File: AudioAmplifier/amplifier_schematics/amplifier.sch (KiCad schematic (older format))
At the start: 2 parts

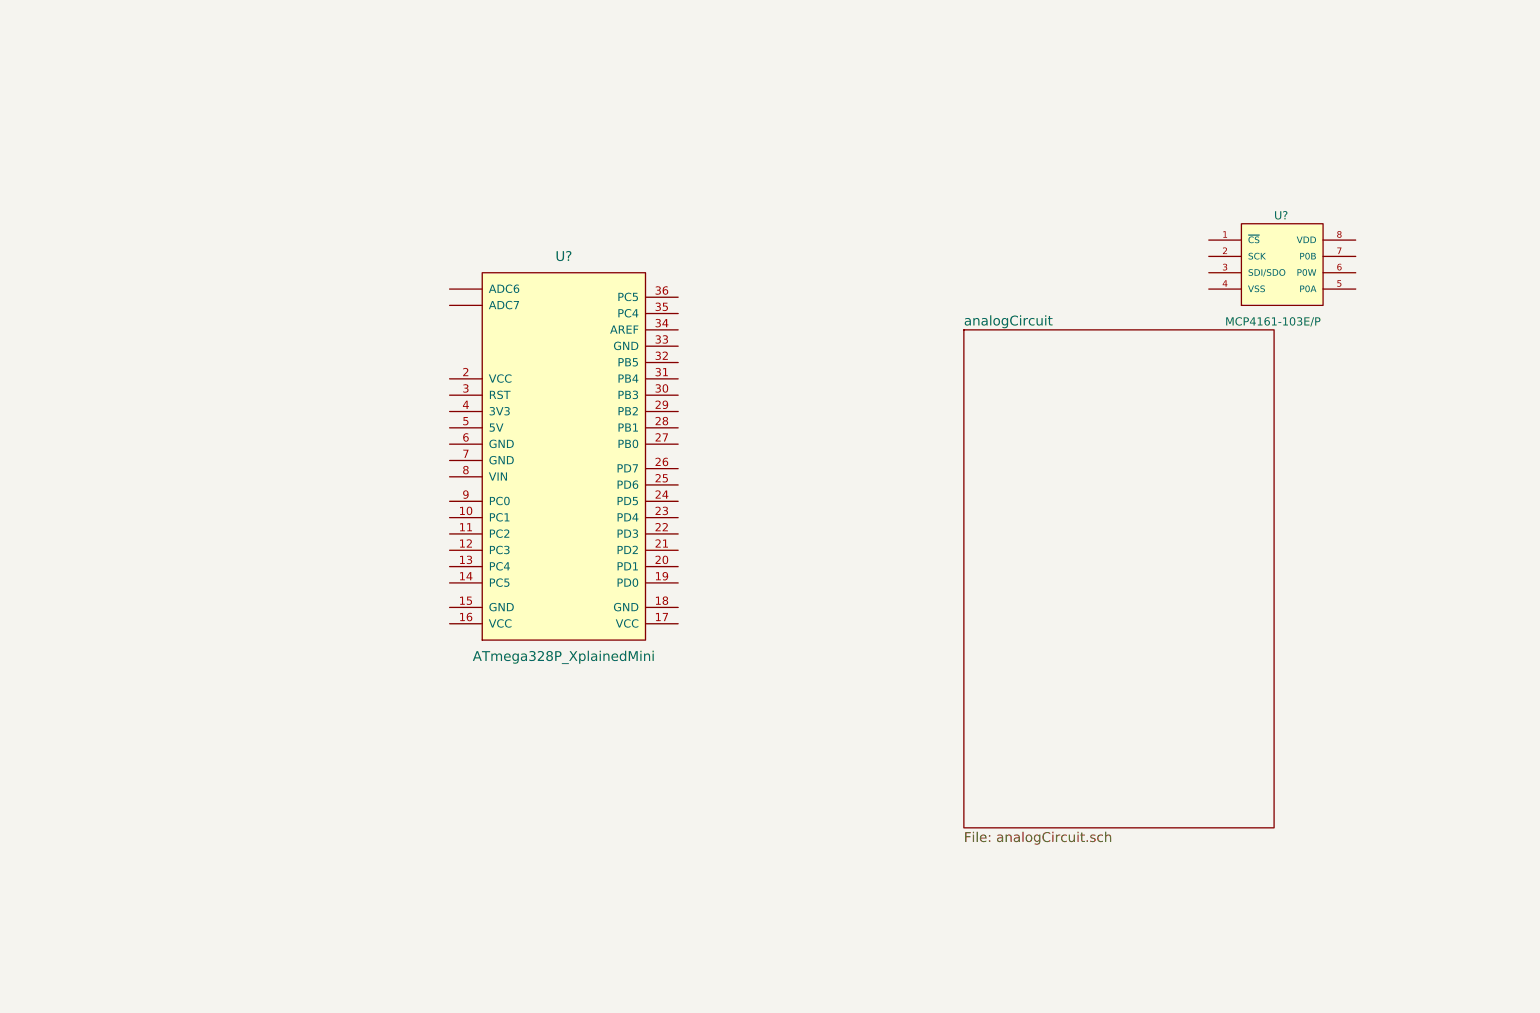
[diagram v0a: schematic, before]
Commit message: updated kicad file
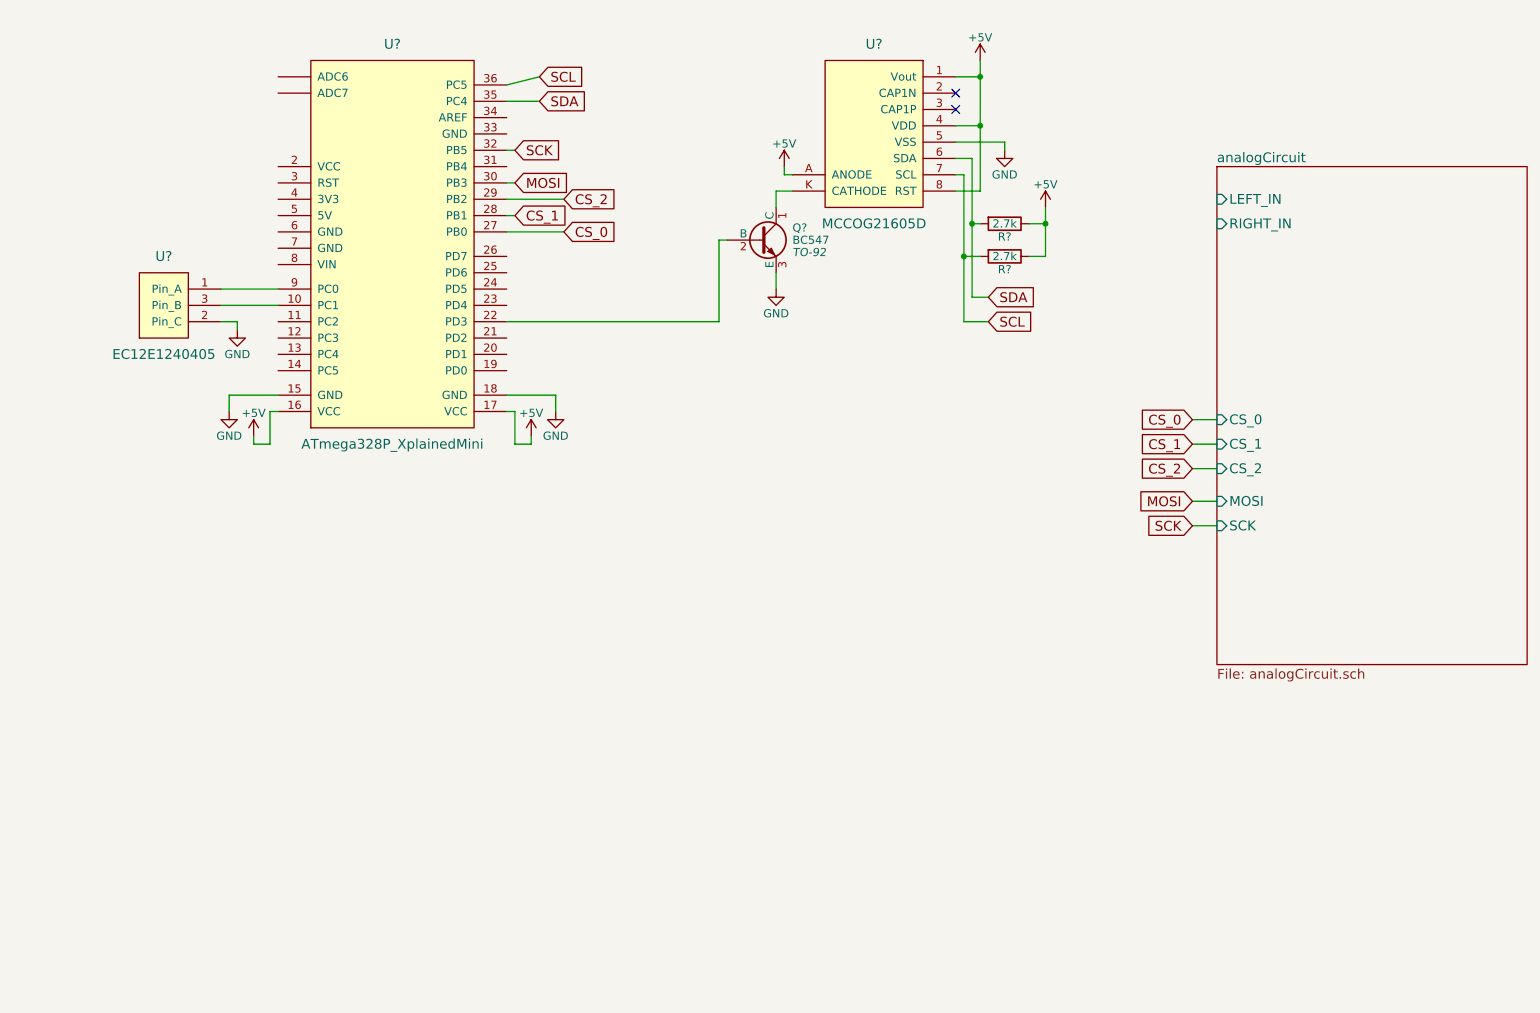
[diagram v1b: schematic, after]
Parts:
- removed U?: MCP4161-103E/P, DIP254P762X533-8, symbol MCP4161-103E/P
- added Q?: BC547, TO-92, symbol BC547
- added R? (x2): 2.7k, symbol R
- added U?: MCCOG21605D, symbol MCCOG21605D
- added U?: EC12E1240405, symbol EC12E1240405
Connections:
- net at U?.10 (PC1): now also U?.3 (Pin_B)
- net GND: now reaches U?.15 (GND)
- net GND: now also U?.18 (GND), Q?.3 (E), U?.2 (Pin_C), U?.5 (VSS)
- net +5V: now reaches U?.16 (VCC)
- net +5V: now also U?.17 (VCC), R?.1, R?.1, U?.1 (Vout), U?.4 (VDD), U?.8 (RST), U?.A (ANODE)
- net at U?.22 (PD3): now also Q?.2 (B)
- net CS_0: now reaches U?.27 (PB0)
- net CS_1: now reaches U?.28 (PB1)
- net CS_2: now reaches U?.29 (PB2)
- net MOSI: now reaches U?.30 (PB3)
- net SCK: now reaches U?.32 (PB5)
- net SDA: now reaches U?.35 (PC4)
- net SDA: now also R?.2, U?.6 (SDA)
- net SCL: now reaches U?.36 (PC5)
- net SCL: now also R?.2, U?.7 (SCL)
- net at U?.9 (PC0): now also U?.1 (Pin_A)
- new net: Q?.1 (C), U?.K (CATHODE)
- no-connect marks 0 -> 2
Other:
- moved on the sheet: U?

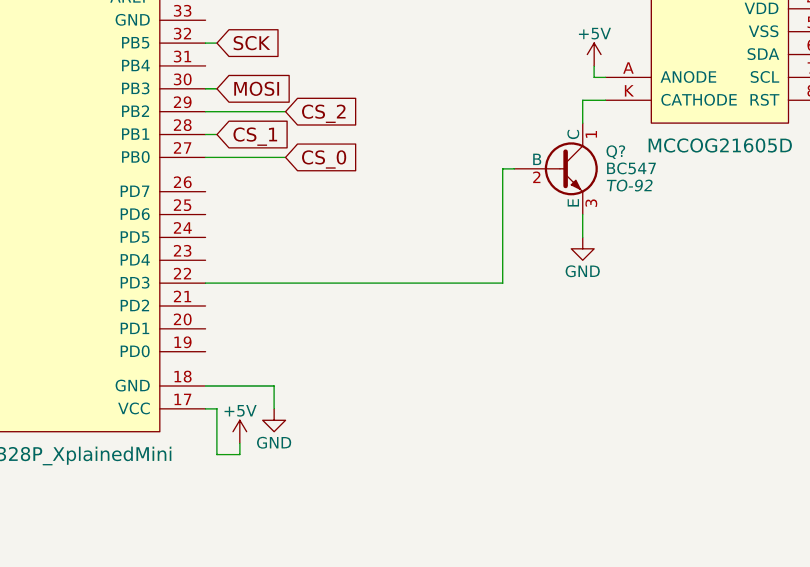
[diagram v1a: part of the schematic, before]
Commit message: kicad schem
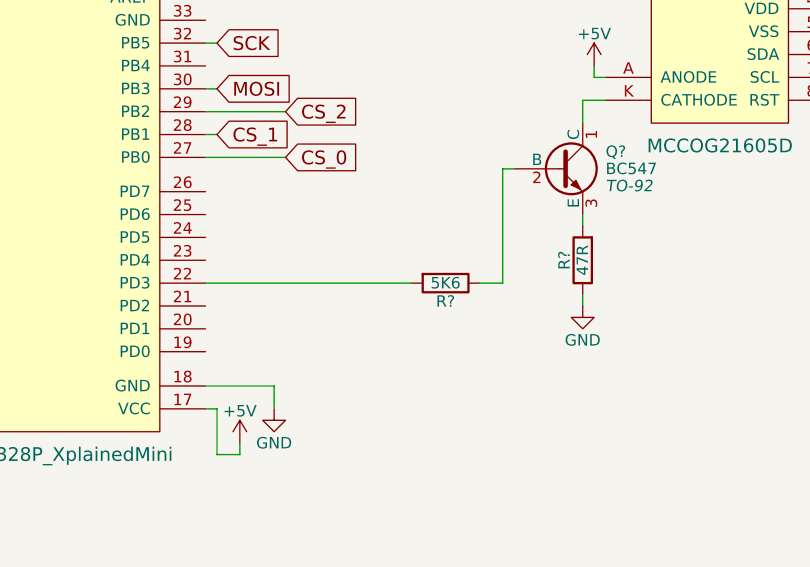
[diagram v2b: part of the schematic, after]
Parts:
- added R?: 5K6, symbol R
- added R?: 47R, symbol R
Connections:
- net GND: now also R?.1; no longer Q?.3 (E)
- net at U?.22 (PD3): now also R?.2; no longer Q?.2 (B)
- new net: Q?.2 (B), R?.1
- new net: Q?.3 (E), R?.2
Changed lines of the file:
@@
 L GND #PWR?
 U 1 1 58FDA342
-P 5200 2900
-F 0 "#PWR?" H 5200 2650 50  0001 C CNN
-F 1 "GND" H 5200 2750 50  0000 C CNN
-F 2 "" H 5200 2900 50  0000 C CNN
-F 3 "" H 5200 2900 50  0000 C CNN
-	1    5200 2900
-	1    0    0    -1
-$EndComp
-Wire Wire Line
-	5200 2800 5200 2900
-Wire Wire Line
-	3550 3100 4850 3100
+P 5200 3200
+F 0 "#PWR?" H 5200 2950 50  0001 C CNN
+F 1 "GND" H 5200 3050 50  0000 C CNN
+F 2 "" H 5200 3200 50  0000 C CNN
+F 3 "" H 5200 3200 50  0000 C CNN
+	1    5200 3200
+	1    0    0    -1
+$EndComp
+Wire Wire Line
+	5200 2800 5200 2850
 Wire Wire Line
 	4850 3100 4850 2600
@@
 Wire Wire Line
 	7750 4350 7900 4350
+$Comp
+L R R?
+U 1 1 5900779A
+P 4600 3100
+F 0 "R?" V 4680 3100 50  0000 C CNN
+F 1 "5K6" V 4600 3100 50  0000 C CNN
+F 2 "" V 4530 3100 50  0000 C CNN
+F 3 "" H 4600 3100 50  0000 C CNN
+	1    4600 3100
+	0    1    1    0
+$EndComp
+$Comp
+L R R?
+U 1 1 5900780C
+P 5200 3000
+F 0 "R?" V 5280 3000 50  0000 C CNN
+F 1 "47R" V 5200 3000 50  0000 C CNN
+F 2 "" V 5130 3000 50  0000 C CNN
+F 3 "" H 5200 3000 50  0000 C CNN
+	1    5200 3000
+	-1   0    0    1
+$EndComp
+Wire Wire Line
+	4750 3100 4850 3100
+Wire Wire Line
+	4450 3100 3550 3100
+Wire Wire Line
+	5200 3150 5200 3200
 $EndSCHEMATC

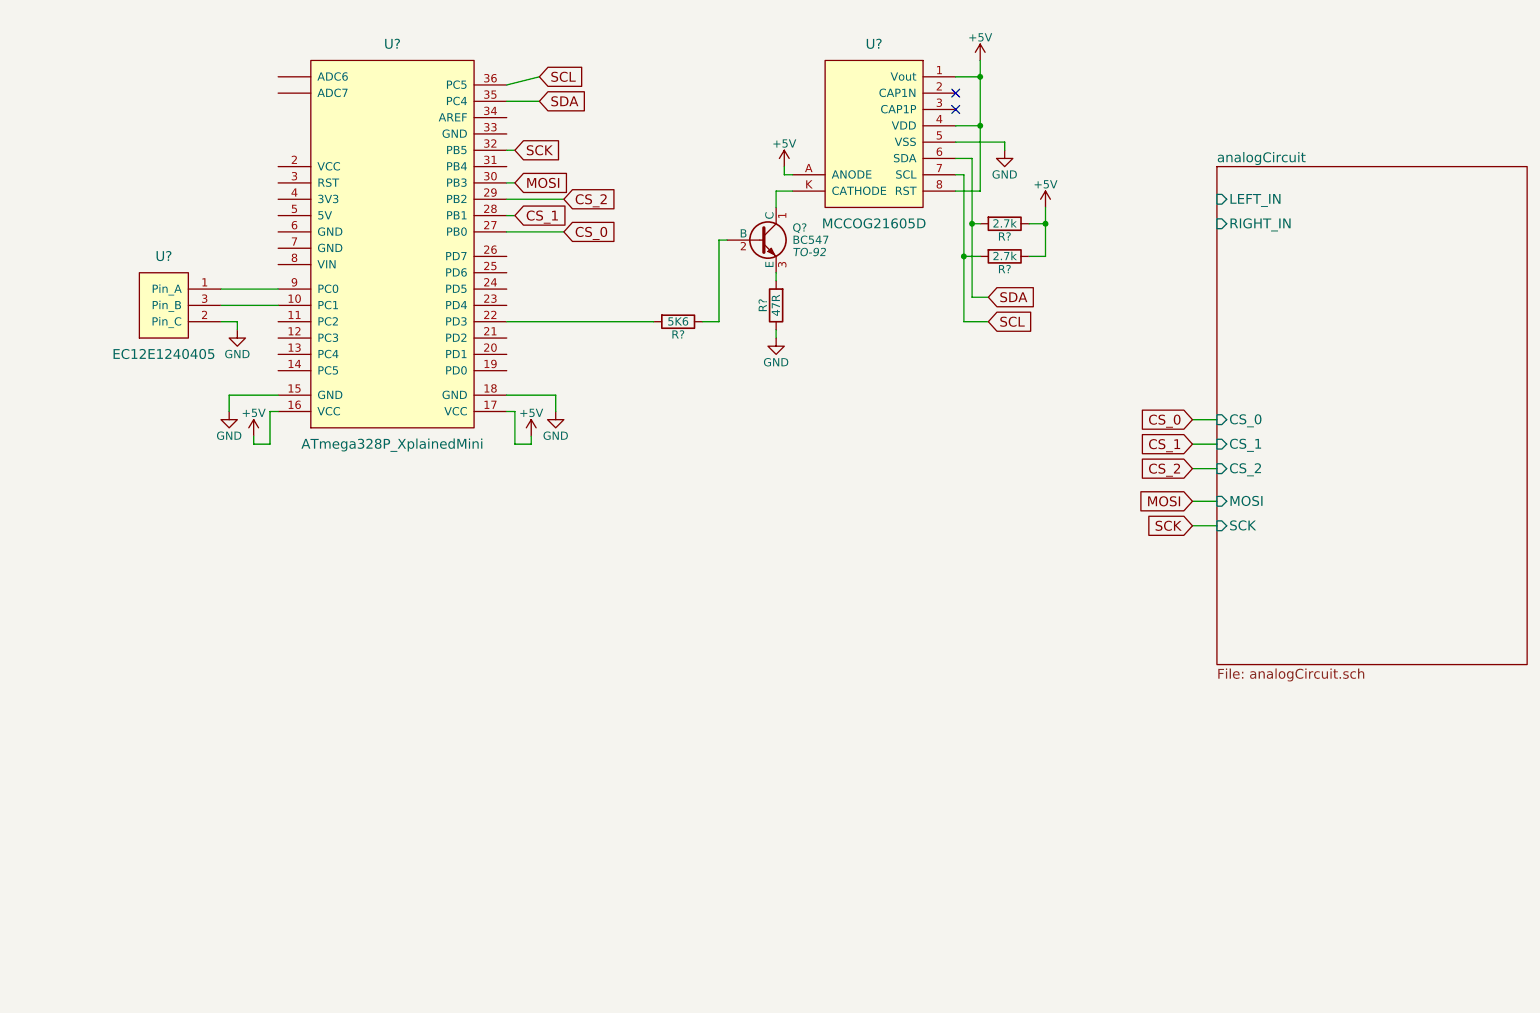
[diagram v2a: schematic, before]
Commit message: kicad
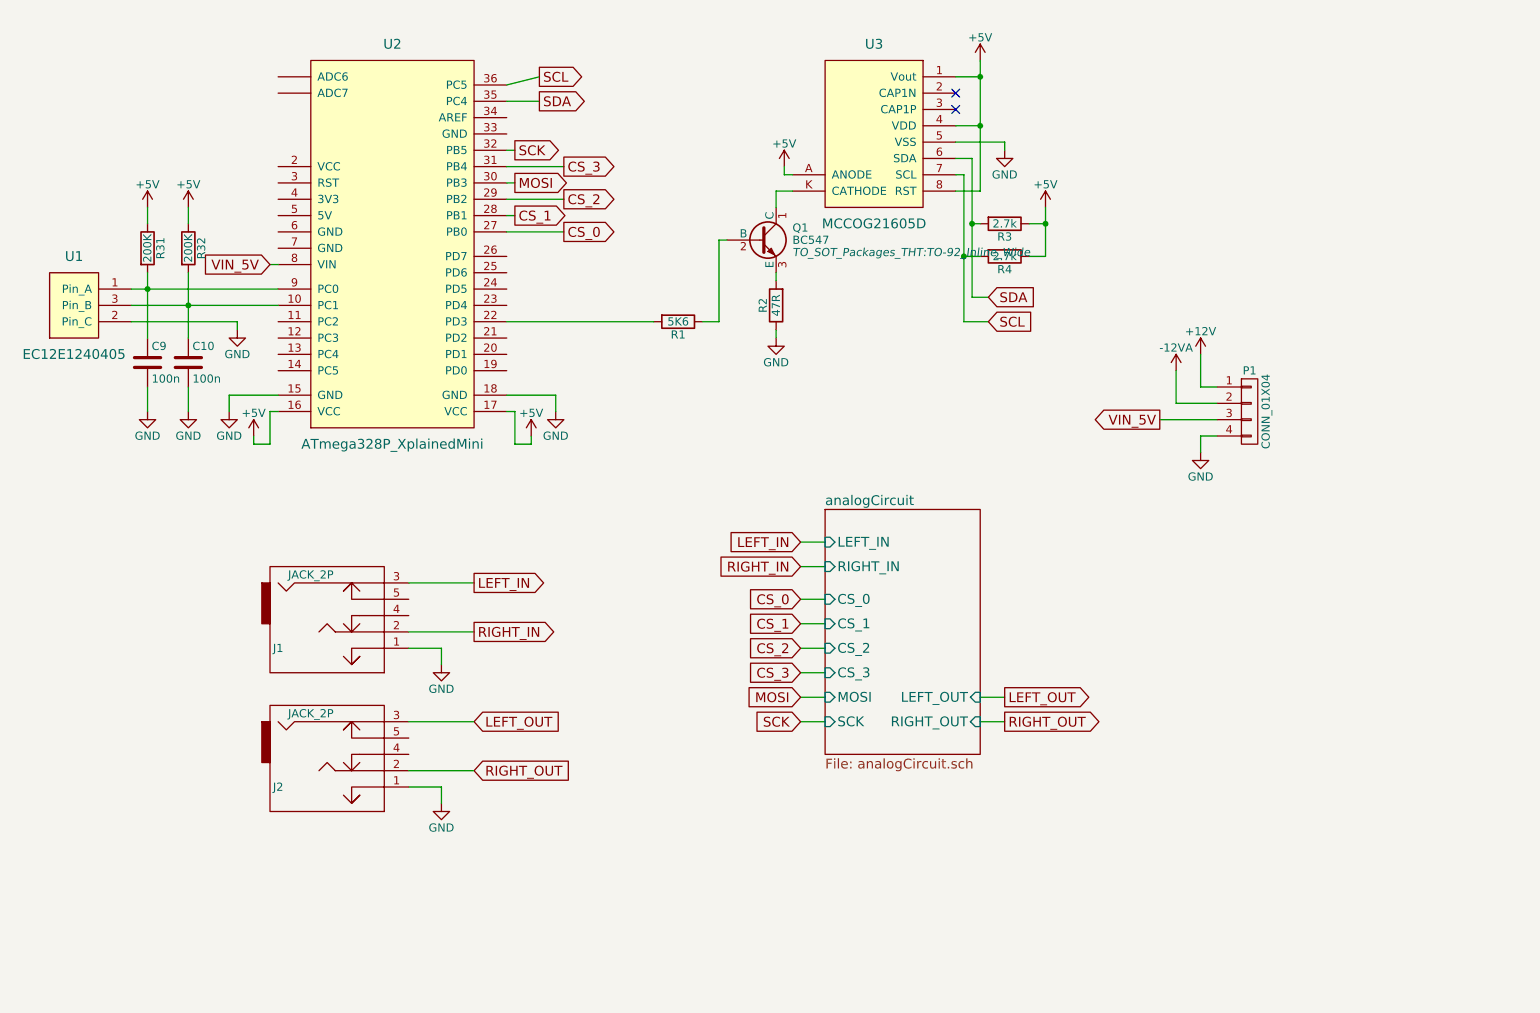
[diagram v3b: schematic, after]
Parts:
- added C10, C9: 100n, Capacitors_THT:C_Disc_D3.0mm_W1.6mm_P2.50mm, symbol C
- added J1, J2: JACK_2P, conektor:JACK_3,5mm_5pin, symbol JACK_2P
- added P1: CONN_01X04, Connectors_Terminal_Blocks:TerminalBlock_Pheonix_MKDS1.5-4pol, symbol CONN_01X04
- added R31, R32: 200K, Resistors_THT:R_Axial_DIN0207_L6.3mm_D2.5mm_P10.16mm_Horizontal, symbol R
- Q1: renamed from Q?; footprint TO-92 -> TO_SOT_Packages_THT:TO-92_Inline_Wide
- R1, R2, R3, R4: renamed from R?; footprint (none) -> Resistors_THT:R_Axial_DIN0207_L6.3mm_D2.5mm_P10.16mm_Horizontal
- U1: renamed from U?; footprint (none) -> rotary:Encoder EC12E
- U2: renamed from U?; footprint (none) -> xplainedBrd:xplained_board
- U3: renamed from U?; footprint (none) -> LCD:MCCOG21605D
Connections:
- net +5V: now also R31.1, R32.1
- net GND: now also C10.2, C9.2, J1.1, J2.1, P1.4 (P4)
- net at U1.3 (Pin_B), U2.10 (PC1): now also C10.1, R32.2
- net CS_3: now reaches U2.31 (PB4)
- net VIN_5V: now reaches U2.8 (VIN)
- net VIN_5V: now also P1.3 (P3)
- net at U1.1 (Pin_A), U2.9 (PC0): now also C9.1, R31.2
- new net +12V: P1.1 (P1)
- new net -12VA: P1.2 (P2)
- new net LEFT_IN: J1.3
- new net LEFT_OUT: J2.3
- new net RIGHT_IN: J1.2
- new net RIGHT_OUT: J2.2
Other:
- moved on the sheet: U1

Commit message: updated KICAD
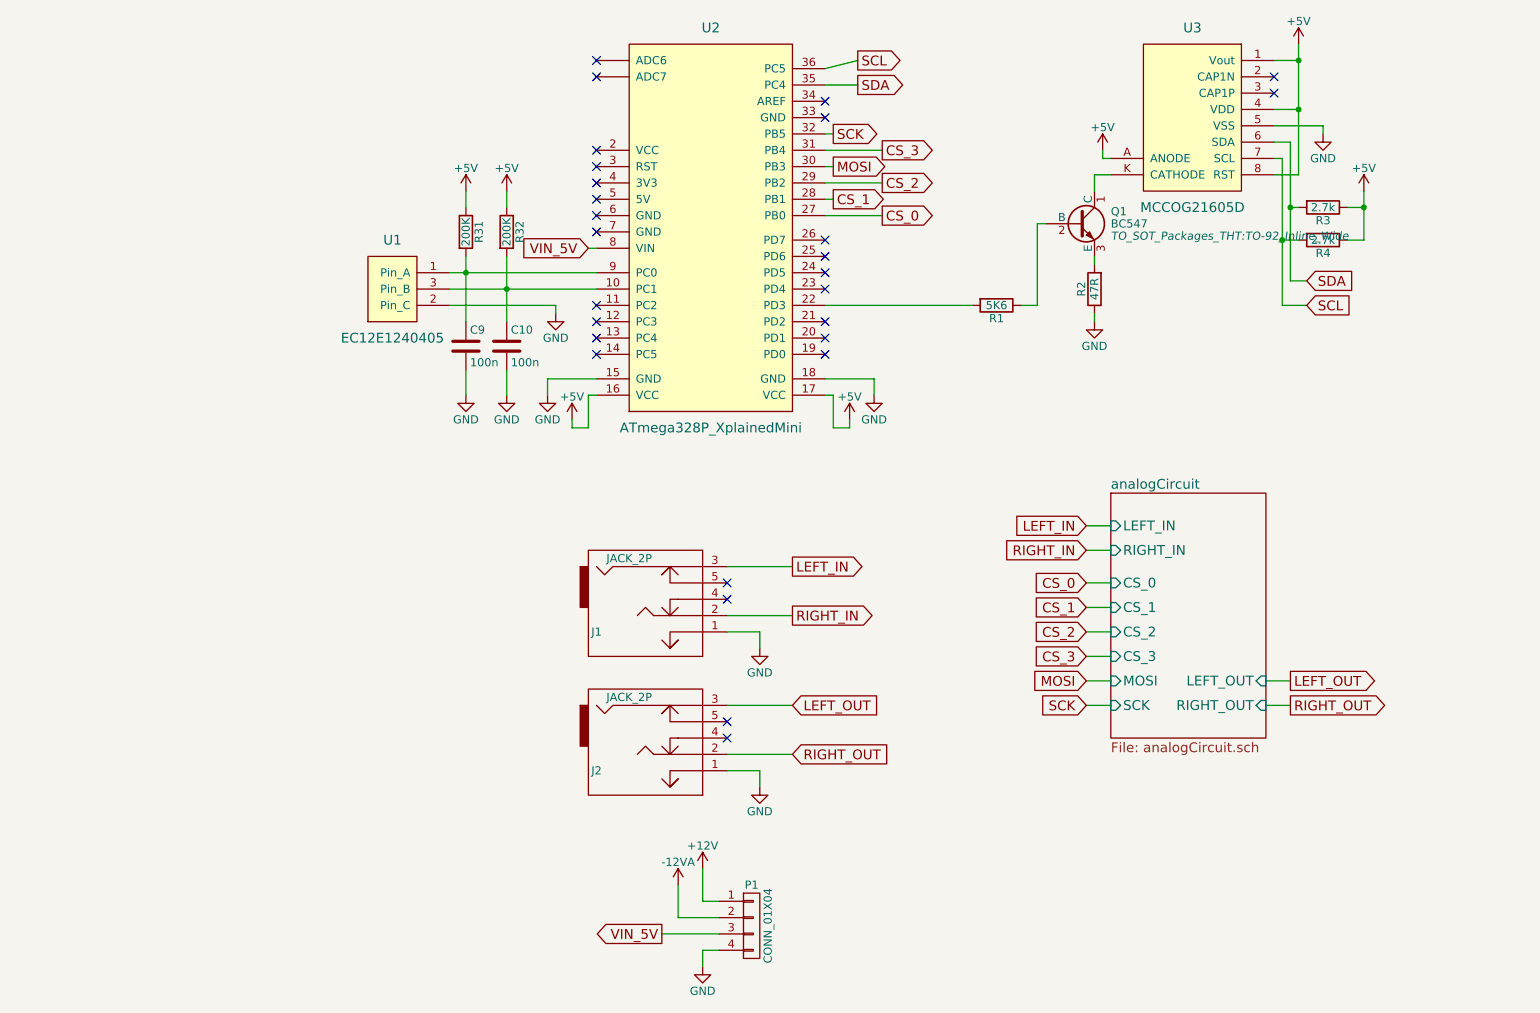
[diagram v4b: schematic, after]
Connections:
- no-connect marks 2 -> 27
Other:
- moved on the sheet: C10, C9, J1, J2, P1, Q1, R1, R2, R3, R31, R32, R4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
